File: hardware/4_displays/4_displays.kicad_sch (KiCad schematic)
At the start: 22 parts, among them J1 Conn_01x08_Male, J2 Conn_01x08_Male, J3 Conn_01x02_Male, Q1 BC807, Q2 BC807, Q3 BC807, Q4 BC807, U1 LTC-4627JG

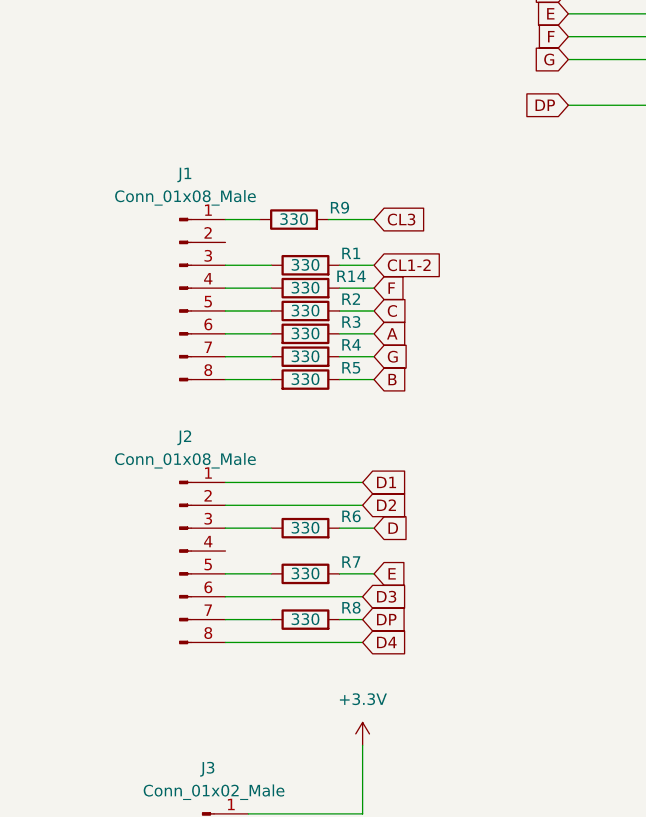
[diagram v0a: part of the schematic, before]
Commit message: Correção do esquemático
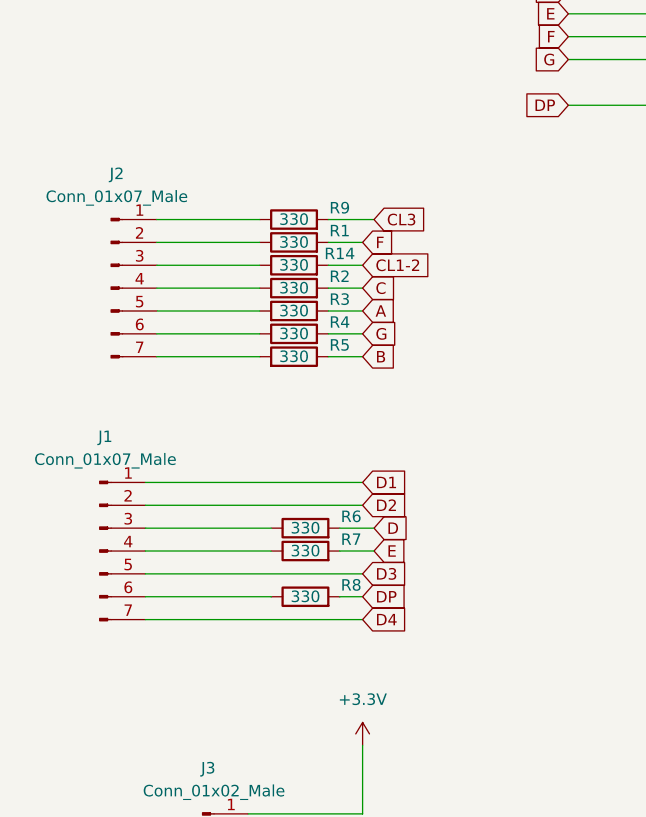
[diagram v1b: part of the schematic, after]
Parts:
- removed J1, J2: Conn_01x08_Male, Connector_PinHeader_2.54mm:PinHeader_1x08_P2.54mm_Vertical, symbol Connector:Conn_01x08_Male
- added J1, J2: Conn_01x07_Male, Connector_PinHeader_2.54mm:PinHeader_1x07_P2.54mm_Vertical, symbol Connector:Conn_01x07_Male
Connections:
- net CL1-2: now also R14.2; no longer R1.2
- net D1: now also J1.1 (Pin_1)
- net D2: now also J1.2 (Pin_2)
- net D3: now also J1.5 (Pin_5)
- net D4: now also J1.7 (Pin_7)
- net F: now also R1.2; no longer R14.2
- net at R6.1: now also J1.3 (Pin_3)
- net at R14.1: now also J2.3 (Pin_3)
- net at R7.1: now also J1.4 (Pin_4)
- net at R8.1: now also J1.6 (Pin_6)
- net at R9.1: now also J2.1 (Pin_1)
- net at R1.1: now also J2.2 (Pin_2)
- net at R2.1: now also J2.4 (Pin_4)
- net at R3.2: now also J2.5 (Pin_5)
- net at R4.1: now also J2.6 (Pin_6)
- net at R5.2: now also J2.7 (Pin_7)
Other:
- moved on the sheet: R1, R14, R2, R3, R4, R5, R7, R8
